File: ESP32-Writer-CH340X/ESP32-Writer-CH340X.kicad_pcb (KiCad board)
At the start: 2 copper layers, 7 parts, among them J1 ESP-Prog-ProgramCOM-SEND, J2 USB2.0_C_v3, U1 CH340X

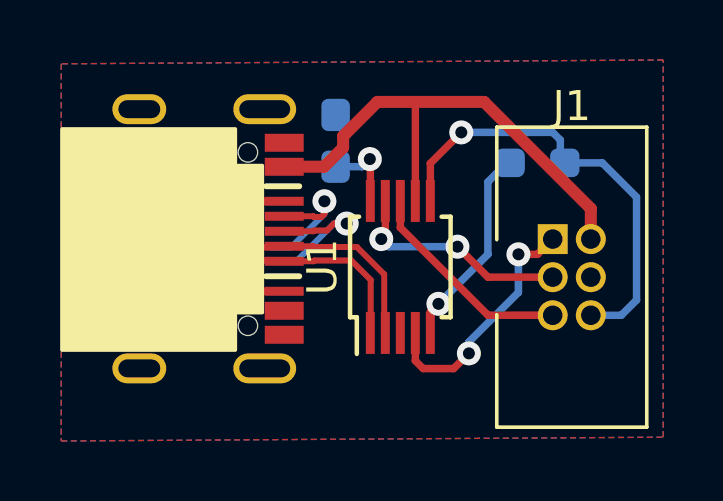
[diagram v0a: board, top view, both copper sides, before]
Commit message: ESP32-Writer-CH340X/v1.0.0
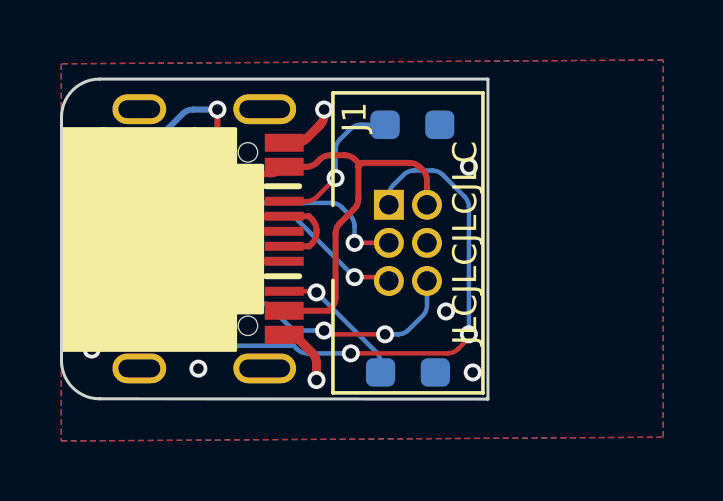
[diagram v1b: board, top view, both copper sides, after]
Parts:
- added G***: LOGO, $74th:74th-4mm, B.Cu at (108.5, 56.5)
- added REF**: JLCJLCJLCJLC, $74th:JLCJLCJLCJLC, F.Cu at (113.9, 58.5)
- added REF**: twitter, $74th:twitter, B.Cu at (111.1, 60.5)
- U1: moved to B.Cu
- moved R3 15.5 mm to (101.3, 59.9), turned to -90 degrees
- moved R2 9.57 mm to (112.2, 54.6), turned to 0 degrees
- moved R1 9.49 mm to (112.0, 62.9), turned to 0 degrees
- moved C2 8.35 mm to (101.3, 56.5), turned to -90 degrees
- moved U1 7.80 mm to (104.0, 58.4)
- moved J1 5.58 mm to (112.0, 58.5)
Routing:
- net EN: track 8.37 -> 20.2 mm
- net GND: track 0.00 -> 8.75 mm, vias 0 -> 11
- net D+: track 15.0 -> 6.83 mm, vias 2 -> 1
- net D-: track 15.0 -> 8.56 mm, vias 2 -> 1
- net Net-(U1-CTS): track 6.83 -> 1.74 mm, vias 1 -> 0
- net +5V: track 17.1 -> 20.5 mm, vias 0 -> 1
- net IO0: track 15.0 -> 17.8 mm, vias 1 -> 5
- net Net-(U1-V3): track 2.65 -> 5.27 mm, vias 1 -> 2
- net TXD: track 7.18 -> 9.33 mm, vias 0 -> 1
- net RXD: track 7.57 -> 8.67 mm, vias 2 -> 1
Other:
- board outline added: 14.2 x 10.7 mm
- board text added: "v1.0.0"
